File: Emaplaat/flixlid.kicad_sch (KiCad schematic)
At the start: 1 part, among them U2 1EDN7550BXTSA1

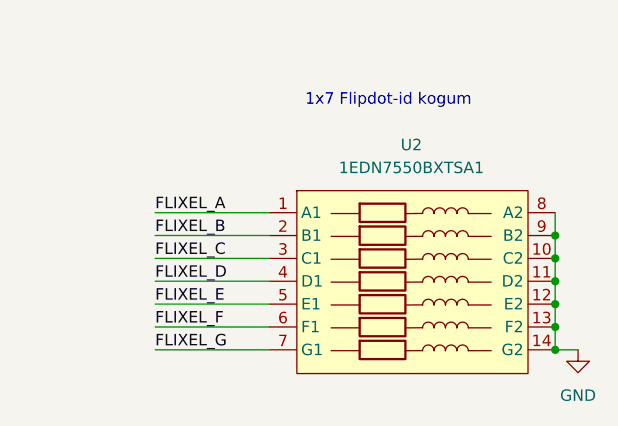
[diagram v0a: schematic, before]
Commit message: uuem versioon
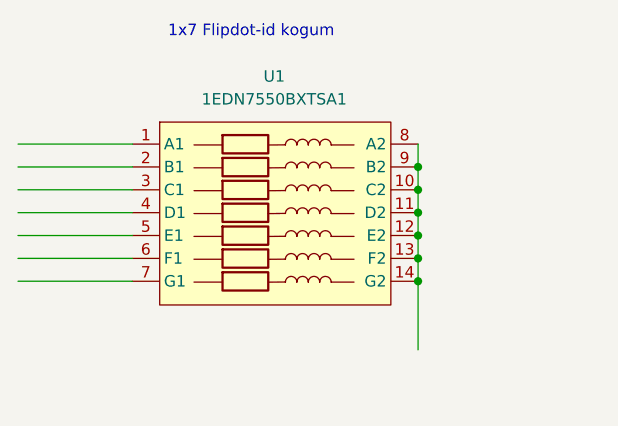
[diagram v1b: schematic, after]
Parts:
- removed U2: 1EDN7550BXTSA1, dot_flipper:7_flip_dots, symbol flipdot_7xarray:flipdot_7xarray
- added U1: 1EDN7550BXTSA1, dot_flipper:7_flip_dots, symbol flipdot_7xarray:flipdot_7xarray
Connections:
- new net: U1.10 (C2), U1.11 (D2), U1.12 (E2), U1.13 (F2), U1.14 (G2), U1.8 (A2), U1.9 (B2)
